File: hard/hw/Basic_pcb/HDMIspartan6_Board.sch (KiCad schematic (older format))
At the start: 50 parts

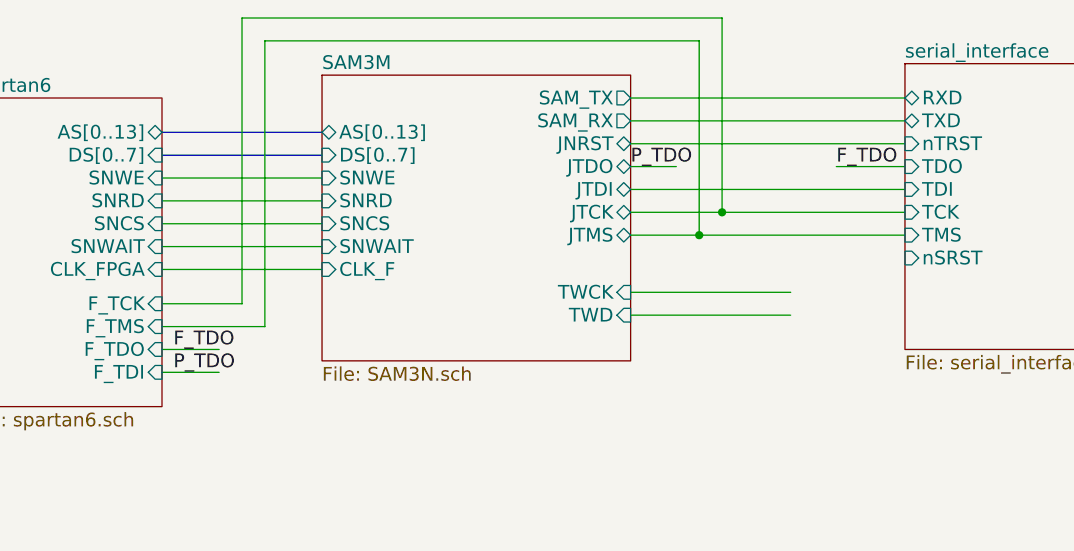
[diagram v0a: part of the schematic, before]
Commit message: ok
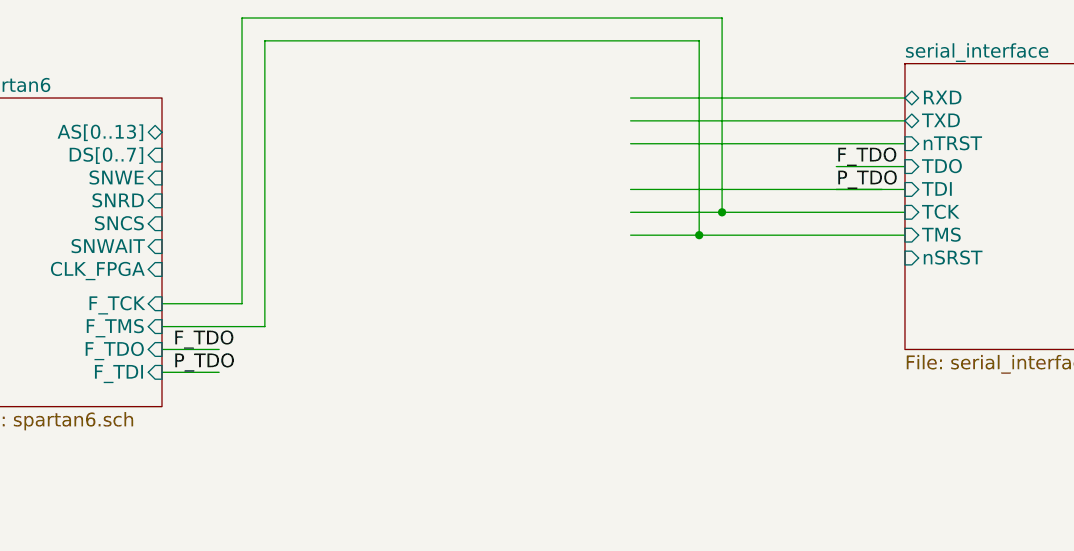
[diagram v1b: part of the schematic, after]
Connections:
- wire segments 30 -> 23
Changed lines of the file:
@@
 EESchema Schematic File Version 2
-LIBS:i.MX283_Board-rescue
 LIBS:power
 LIBS:device
@@
 LIBS:lan8720a
 LIBS:rj45_stamp
-LIBS:i.MX283_Board-cache
+LIBS:HDMIspartan6_Board-cache
 EELAYER 25 0
 EELAYER END
@@
 Comment4 ""
 $EndDescr
-$Sheet
-S 4750 3200 1350 1250
-U 4E78AF25
-F0 "SAM3M" 60
-F1 "SAM3N.sch" 60
-F2 "JNRST" B R 6100 3500 60
-F3 "JTMS" B R 6100 3900 60
-F4 "JTCK" B R 6100 3800 60
-F5 "JTDO" B R 6100 3600 60
-F6 "JTDI" B R 6100 3700 60
-F7 "SAM_RX" O R 6100 3400 60
-F8 "SAM_TX" O R 6100 3300 60
-F9 "TWD" I R 6100 4250 60
-F10 "TWCK" I R 6100 4150 60
-F11 "DS[0..7]" I L 4750 3550 60
-F12 "SNWE" I L 4750 3650 60
-F13 "SNRD" I L 4750 3750 60
-F14 "SNCS" I L 4750 3850 60
-F15 "SNWAIT" I L 4750 3950 60
-F16 "AS[0..13]" B L 4750 3450 60
-F17 "CLK_F" I L 4750 4050 60
-$EndSheet
 $Sheet
 S 3200 3300 850  1350
@@
 F12 "CLK_FPGA" I R 4050 4050 60
 $EndSheet
-Text Label 6100 3600 0    60   ~ 0
+Text Label 7000 3700 0    60   ~ 0
 P_TDO
 Text Label 4100 4500 0    60   ~ 0
@@
 	6100 3400 7300 3400
 Wire Wire Line
-	6800 4250 6100 4250
-Wire Wire Line
 	6100 3500 7300 3500
 Wire Wire Line
@@
 	6100 3900 7300 3900
 Wire Wire Line
-	6100 4150 6800 4150
-Wire Wire Line
 	6100 3300 7300 3300
-Wire Wire Line
-	4050 3650 4750 3650
-Wire Wire Line
-	4050 3750 4750 3750
-Wire Wire Line
-	4050 3850 4750 3850
-Wire Wire Line
-	4050 3950 4750 3950
-Wire Bus Line
-	4050 3450 4750 3450
-Wire Bus Line
-	4050 3550 4750 3550
 Wire Wire Line
 	6500 3800 6500 2950
@@
 	4300 4500 4050 4500
 Wire Wire Line
-	6300 3600 6100 3600
+	7200 3700 7000 3700
 Wire Wire Line
 	6100 3700 7300 3700
-Wire Wire Line
-	4750 4050 4050 4050
 Text Label 7000 3600 0    60   ~ 0
 F_TDO
